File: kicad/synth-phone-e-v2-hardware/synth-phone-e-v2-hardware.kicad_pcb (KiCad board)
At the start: 2 copper layers, 62 x 60 mm, 21 parts, among them J12 display_socket, J15 encoder_input, J16 4P4C, J3 DIN-5, J4 Keypad_column_output, J5 Jack-in, J6 keypad socket, J7 keypad_row_output, J8 jack-out, SW13 SW_Wuerth_450301014042, SW14 SW_Push_SPDT, U2 6N138

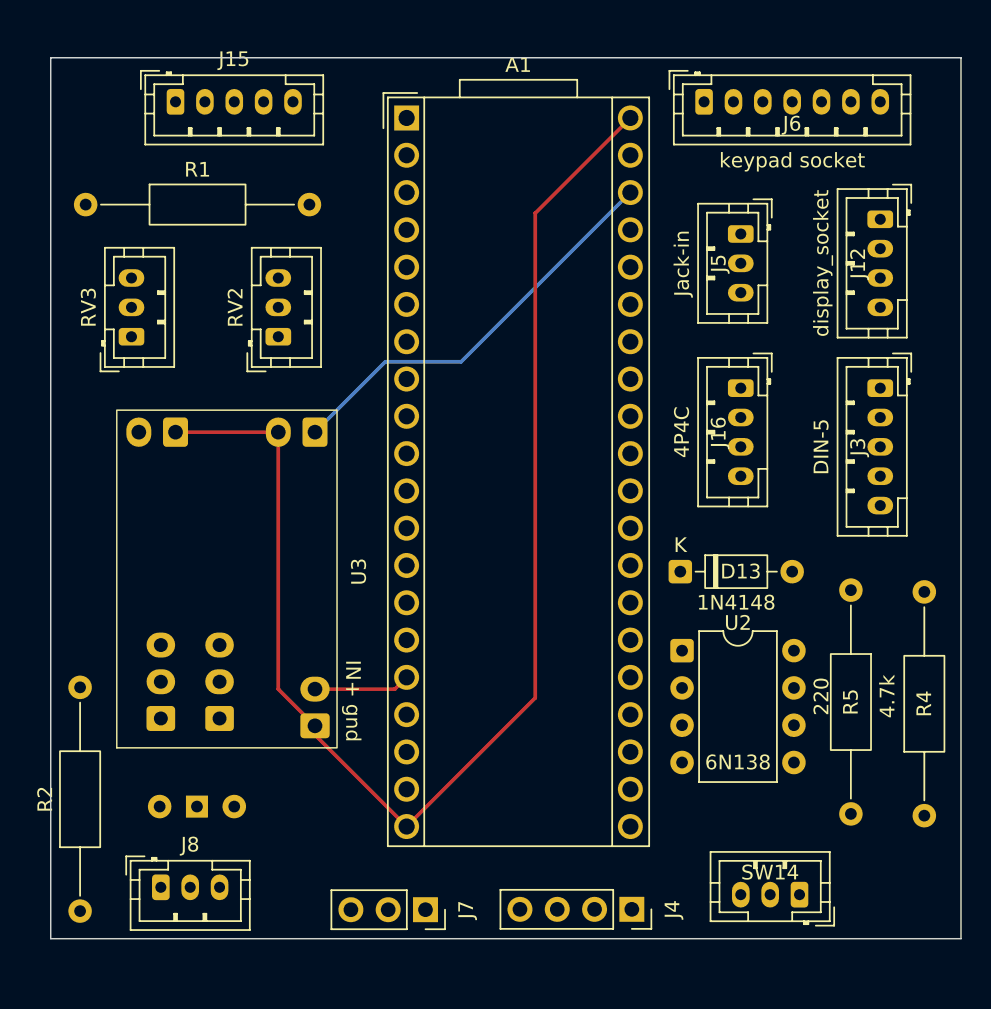
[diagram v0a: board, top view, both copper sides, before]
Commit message: feat: finish pcb
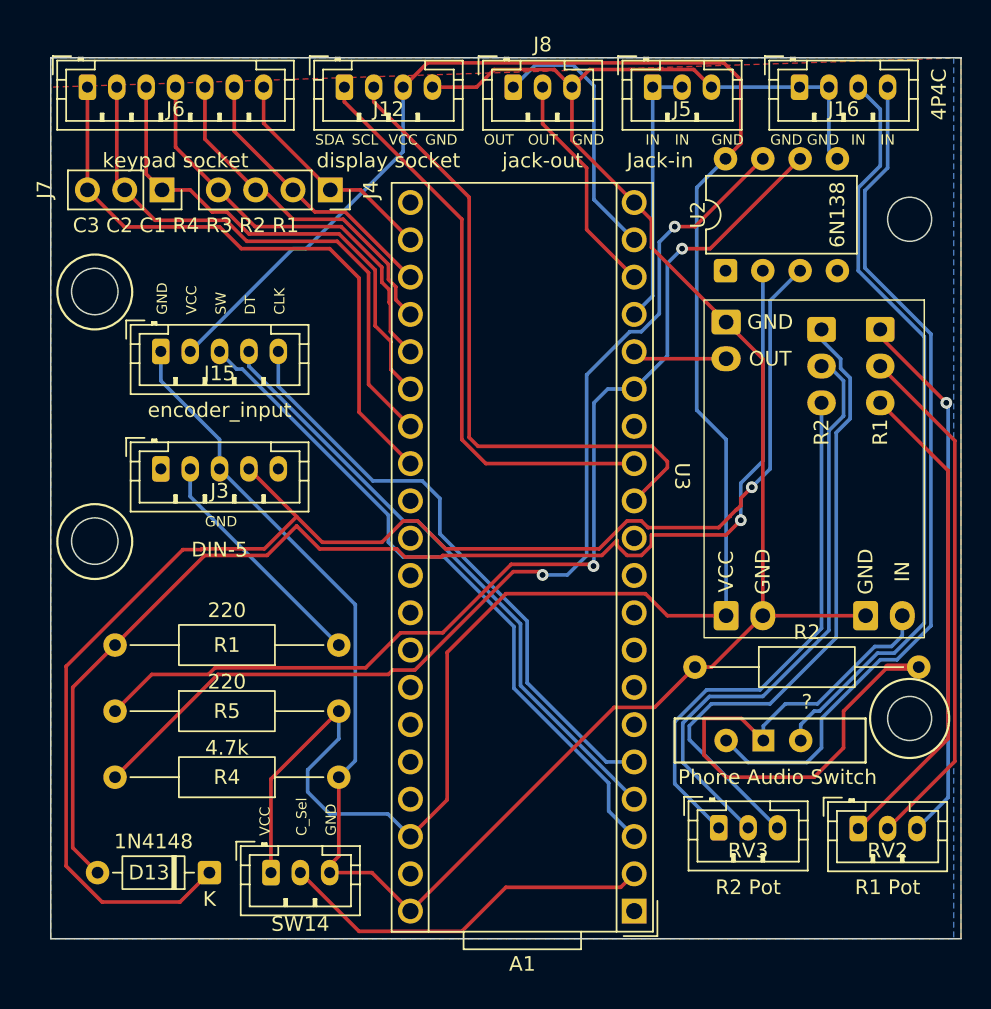
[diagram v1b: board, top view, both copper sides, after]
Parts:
- J12: value display_socket -> display socket
- moved J8 59.6 mm to (43.5, 52.5)
- moved A1 56.2 mm to (51.7, 108.6), turned to 180 degrees
- moved J4 53.1 mm to (31.0, 59.5)
- moved J7 52.2 mm to (19.6, 59.5)
- moved RV3 52.1 mm to (57.5, 103.0), turned to 0 degrees
- moved RV2 51.8 mm to (67.0, 103.0), turned to 0 degrees
- moved R5 50.8 mm to (16.4, 95.0), turned to 0 degrees
- moved J3 49.3 mm to (19.5, 78.5), turned to 0 degrees
- moved R2 45.1 mm to (55.9, 92.0), turned to 0 degrees
- moved J6 42.0 mm to (14.5, 52.5)
- moved U3 40.5 mm to (64.0, 79.0), turned to -90 degrees
- moved R4 40.0 mm to (31.6, 99.5), turned to 180 degrees
- moved SW13 38.8 mm to (60.5, 97.0)
- moved D13 38.1 mm to (22.8, 106.0), turned to 180 degrees
- moved J12 37.6 mm to (32.0, 52.5), turned to 0 degrees
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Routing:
- net vcc: track 28.2 -> 149.7 mm
- net Net-(D13-K): track 0.00 -> 101.4 mm, vias 0 -> 1
- net Net-(D13-A): track 0.00 -> 84.4 mm, vias 0 -> 1
- net MIDI_in_device: track 0.00 -> 72.5 mm, vias 0 -> 2
- net Net-(U2-VO1): track 0.00 -> 71.8 mm, vias 0 -> 2
- net gnd: track 92.1 -> 163.1 mm
- net Net-(SW13-C): track 0.00 -> 58.8 mm
- net Net-(SW13-A): track 0.00 -> 52.0 mm
- net sw: track 0.00 -> 46.6 mm
- net SCL: track 0.00 -> 44.3 mm
- net Net-(U3-R2L): track 0.00 -> 44.1 mm
- net col3: track 0.00 -> 42.1 mm
- net dt: track 0.00 -> 41.9 mm
- net AUDIO_IN_1_4p4c: track 0.00 -> 41.3 mm
- net clk: track 0.00 -> 41.1 mm
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- added copper zone on B.Cu, net gnd
- added copper zone on F.Cu, net gnd
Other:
- outline, holes or cut-outs redrawn
- board text added: "C3 C2 C1 R4 R3 R2 R1"
- board text added: "CLK"
- board text added: "C_Sel"
- board text added: "DT"
- board text added: "GND"
- board text added: "IN"
- board text added: "OUT"
- board text added: "Phone Audio Switch"
- board text added: "R1"
- board text added: "R1 Pot"
- board text added: "R2"
- board text added: "R2 Pot"
- board text added: "SCL"
- board text added: "SDA"
- board text added: "SW"
- board text added: "VCC"
- board text removed: "IN+"
- board text removed: "gnd"
